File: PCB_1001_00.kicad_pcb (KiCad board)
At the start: 2 copper layers, 37.6 x 33.5 mm, 10 parts, among them SW1 SW_MEC_5G, SW2 SW_MEC_5G, SW3 SW_MEC_5G

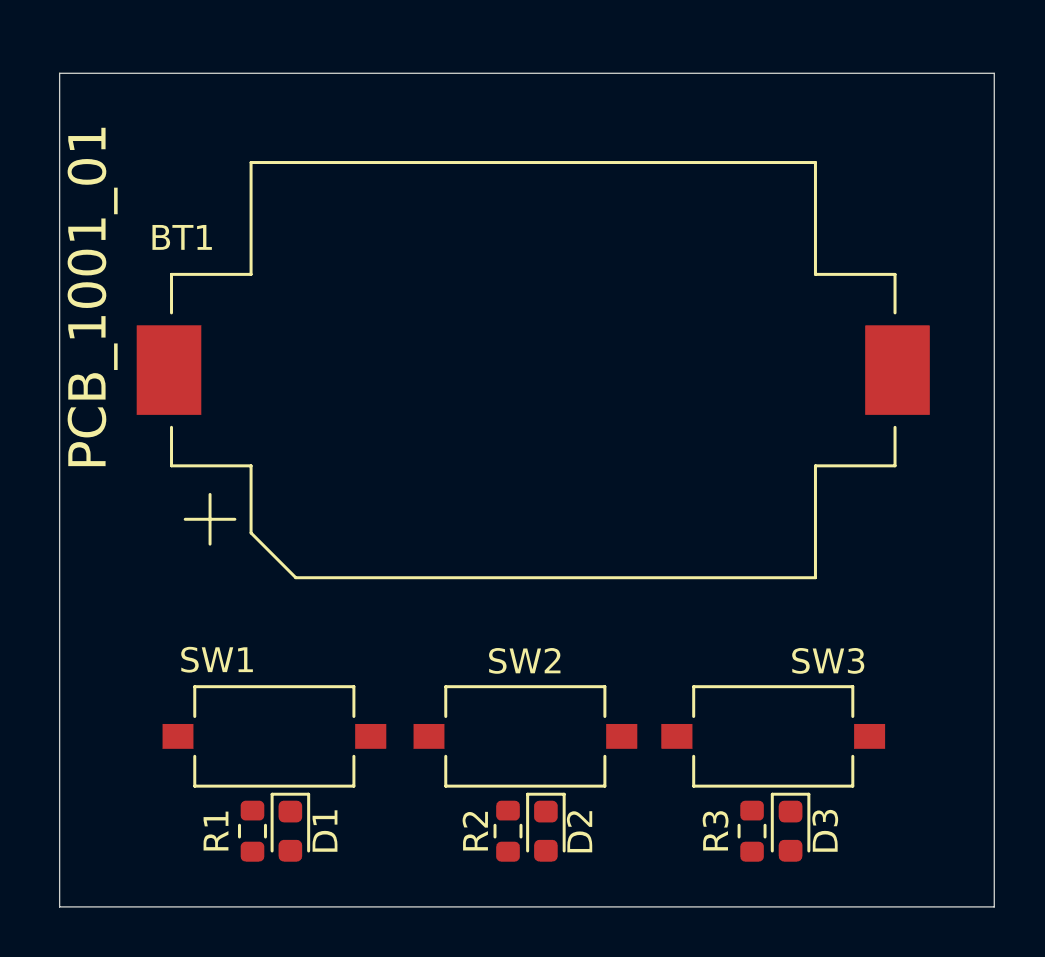
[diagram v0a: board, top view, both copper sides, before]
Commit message: PCB_1001_01 routing completed
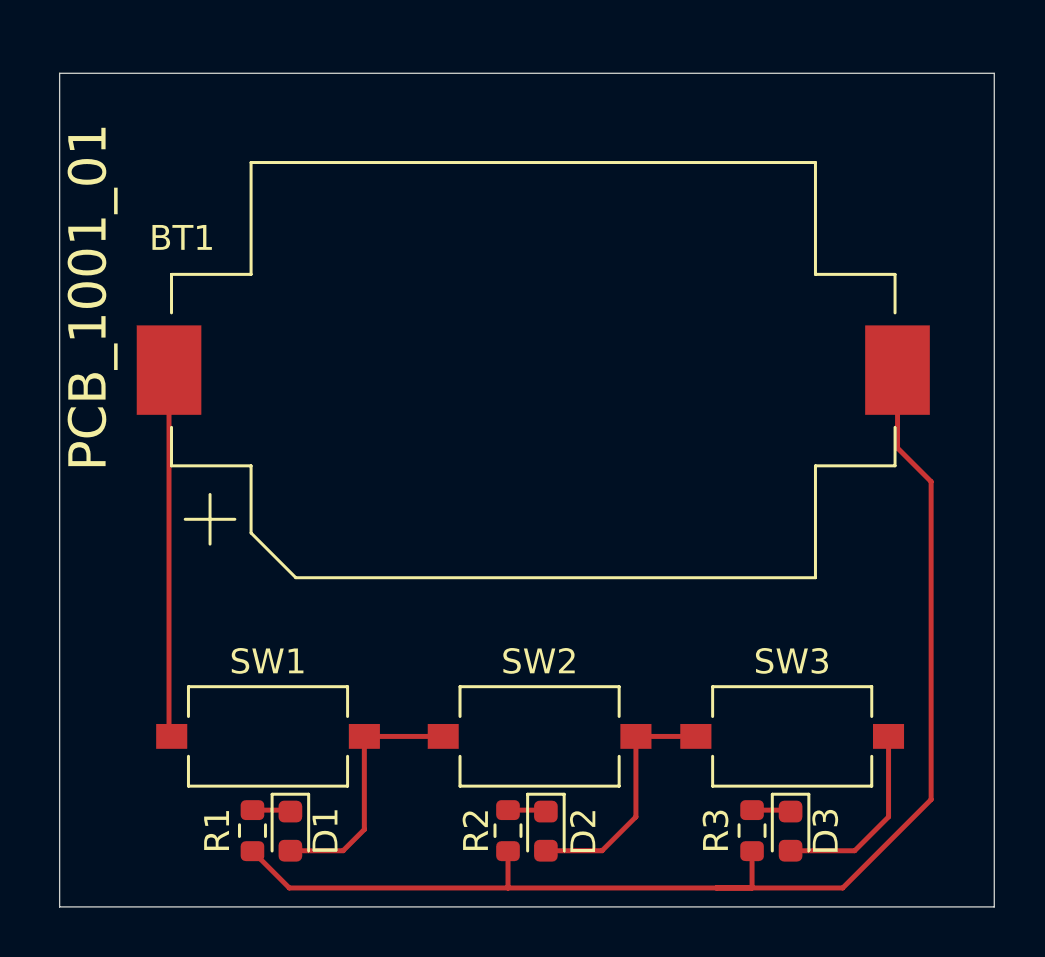
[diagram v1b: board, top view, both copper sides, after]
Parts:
- SW1, SW2, SW3: value SW_MEC_5G -> SW_MEC_5G_edit
- moved SW3 0.76 mm to (153.2, 105.2)
- moved SW2 0.57 mm to (143.0, 105.2)
- moved SW1 0.25 mm to (132.1, 105.2)
- turned R1 to -90 degrees
- turned R2 to -90 degrees
- turned R3 to -90 degrees
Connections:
- SW1 pad 2: Net-(BT1-+) -> Net-(D1-A)
- SW2 pad 2: Net-(D1-A) -> Net-(D2-A)
- SW3 pad 2: Net-(D2-A) -> Net-(D3-A)
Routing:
- net Net-(BT1--): track 0.00 -> 51.6 mm
- net Net-(BT1-+): track 0.00 -> 14.8 mm
- net Net-(D1-A): track 0.00 -> 10.2 mm
- net Net-(D2-A): track 0.00 -> 9.83 mm
- net Net-(D3-A): track 0.00 -> 7.74 mm
- net Net-(D3-K): track 0.00 -> 1.57 mm
- net Net-(D2-K): track 0.00 -> 1.55 mm
- net Net-(D1-K): track 0.00 -> 1.55 mm
